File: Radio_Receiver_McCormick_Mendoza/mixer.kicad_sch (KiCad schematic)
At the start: 32 parts, among them J13 I_0, J14 I_180, J15 Q_90, J16 Q_270, J17 I_RAW, J18 Conn_01x02_Female, J19 Conn_01x02_Female, J20 Q_RAW, U11 INA821ID, U8 SN74CBT3253CDBR, U9 INA821ID

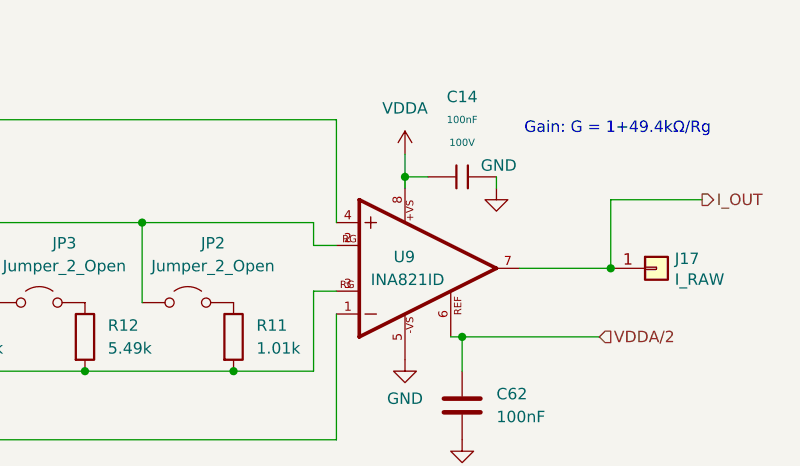
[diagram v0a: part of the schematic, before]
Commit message: Updated footprints
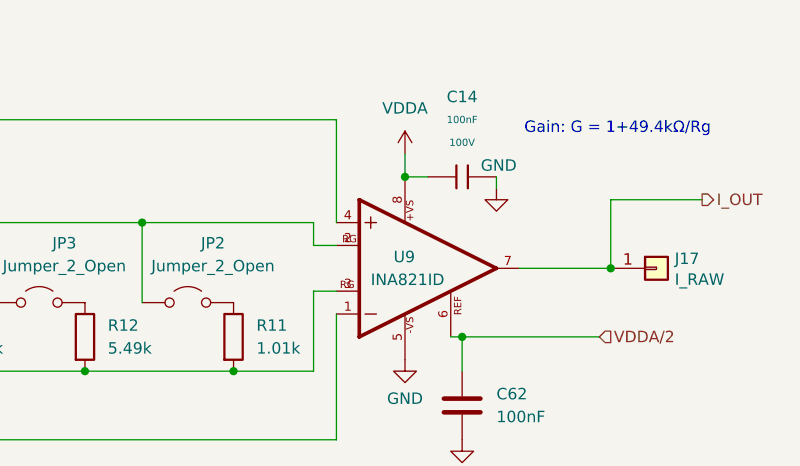
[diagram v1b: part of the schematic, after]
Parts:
- U11, U9: footprint import_footprint:SOIC127P600X175-8N -> INA821ID:D0008A_N
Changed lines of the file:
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@@
 	(wire
 		(pts
-			(xy 238.76 50.8) (xy 238.76 49.53)
-		)
-		(stroke
-			(width 0)
-			(type default)
-		)
-	)
-	(wire
-		(pts
 			(xy 219.71 71.12) (xy 228.6 71.12)
 		)
@@
 			)
 		)
-		(property "Footprint" "import_footprint:SOIC127P600X175-8N"
+		(property "Footprint" "INA821ID:D0008A_N"
 			(at 242.57 123.19 0)
 			(hide yes)
@@
 			)
 		)
-		(property "Footprint" "import_footprint:SOIC127P600X175-8N"
+		(property "Footprint" "INA821ID:D0008A_N"
 			(at 241.3 59.69 0)
 			(hide yes)
